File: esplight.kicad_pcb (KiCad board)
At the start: 2 copper layers, 14 parts, among them P1 CONN_01X03, P2 CONN_01X04, U1 AMS1117, U2 ESP-201

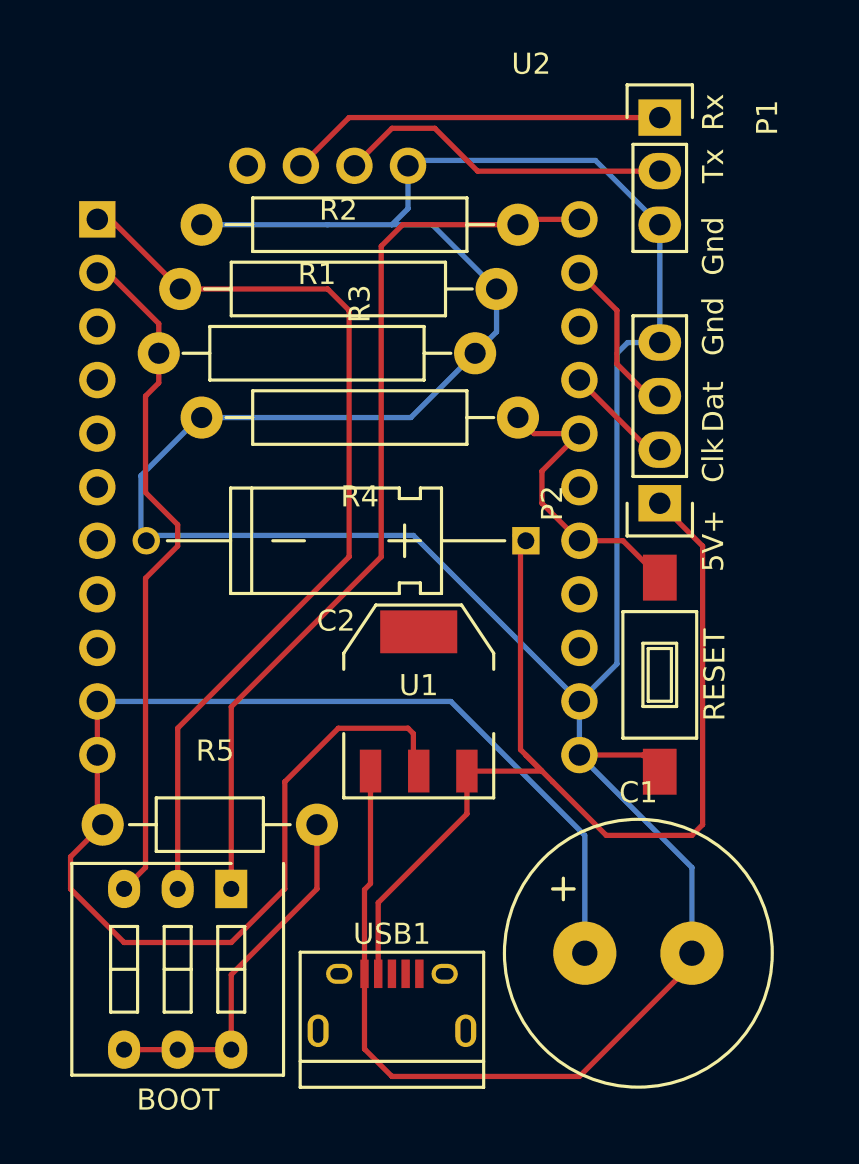
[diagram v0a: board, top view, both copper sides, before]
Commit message: got the board to a more or less finished state - gonna try variants now
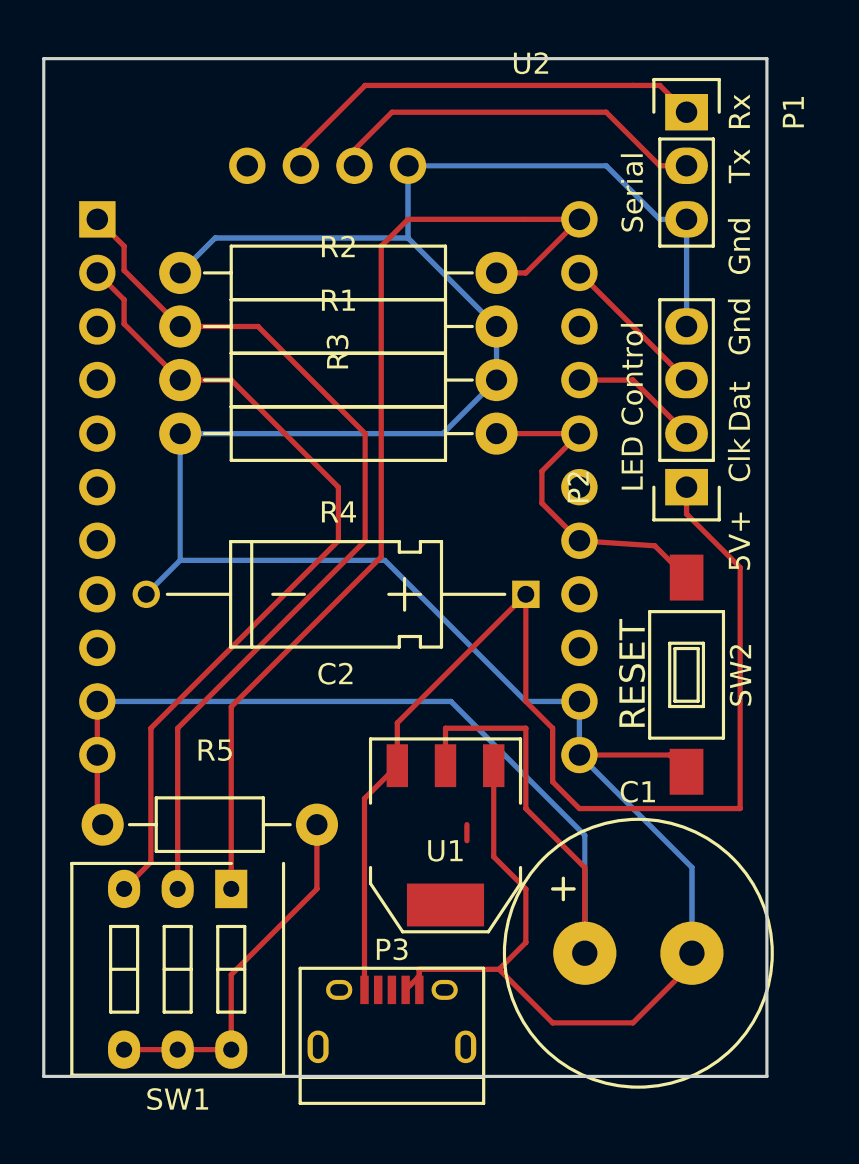
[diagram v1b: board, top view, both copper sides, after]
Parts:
- removed USB1: BARREL_JACK, Connect:USB_Micro-B
- added P3: USB_B, Connect:USB_Micro-B, F.Cu at (27.9, 59.7)
- R1, R2, R3, R4: value 20kE -> 10kE
- SW1: renamed from BOOT; value DIPS_03 -> BOOT
- SW2: renamed from RESET; value SW_PUSH -> RESET
- moved U1 6.48 mm to (30.5, 50.8), turned to 180 degrees
- moved C2 2.54 mm to (34.3, 39.4)
- moved R3 2.50 mm to (25.4, 24.1)
- moved R2 1.78 mm to (25.4, 26.7)
- moved R1 1.63 mm to (25.4, 29.2)
- moved P2 1.48 mm to (41.9, 34.3)
- moved P1 1.30 mm to (41.9, 16.5)
- moved R4 1.27 mm to (25.4, 31.8)
- moved SW2 1.27 mm to (41.9, 43.2)
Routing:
- net GND: track 155.8 -> 137.4 mm
- net /3.3V: track 68.1 -> 55.1 mm
- net Net-(R1-Pad1): track 33.6 -> 40.2 mm
- net Net-(R3-Pad1): track 43.3 -> 48.3 mm
- net /+5V: track 53.0 -> 57.1 mm
- net Net-(P1-Pad1): track 18.0 -> 20.8 mm
- net Net-(P1-Pad2): track 16.1 -> 18.3 mm
- net Net-(R4-Pad1): track 14.3 -> 16.5 mm
- net Net-(R2-Pad1): track 44.5 -> 43.5 mm
- net Net-(P2-Pad2): track 5.18 -> 6.13 mm
- net (no net): track 0.00 -> 0.76 mm
- net Net-(P2-Pad3): track 7.72 -> 7.18 mm
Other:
- board outline added: 34.3 x 48.3 mm
- rule via_min_drill: 0.3 -> 0.35
- board text added: "GPIO 0"
- board text added: "GPIO 2"
- board text added: "GPIO15"
- board text added: "GPIO2 GPIO0 GPIO15 H L L Download H H L Boot Flash X X H Boot SD"
- board text added: "LED Control"
- board text added: "RESET"
- board text added: "Serial"
